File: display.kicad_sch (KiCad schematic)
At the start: 17 parts, among them Q1 ZXM61N03F, U1 E2206KS0E1

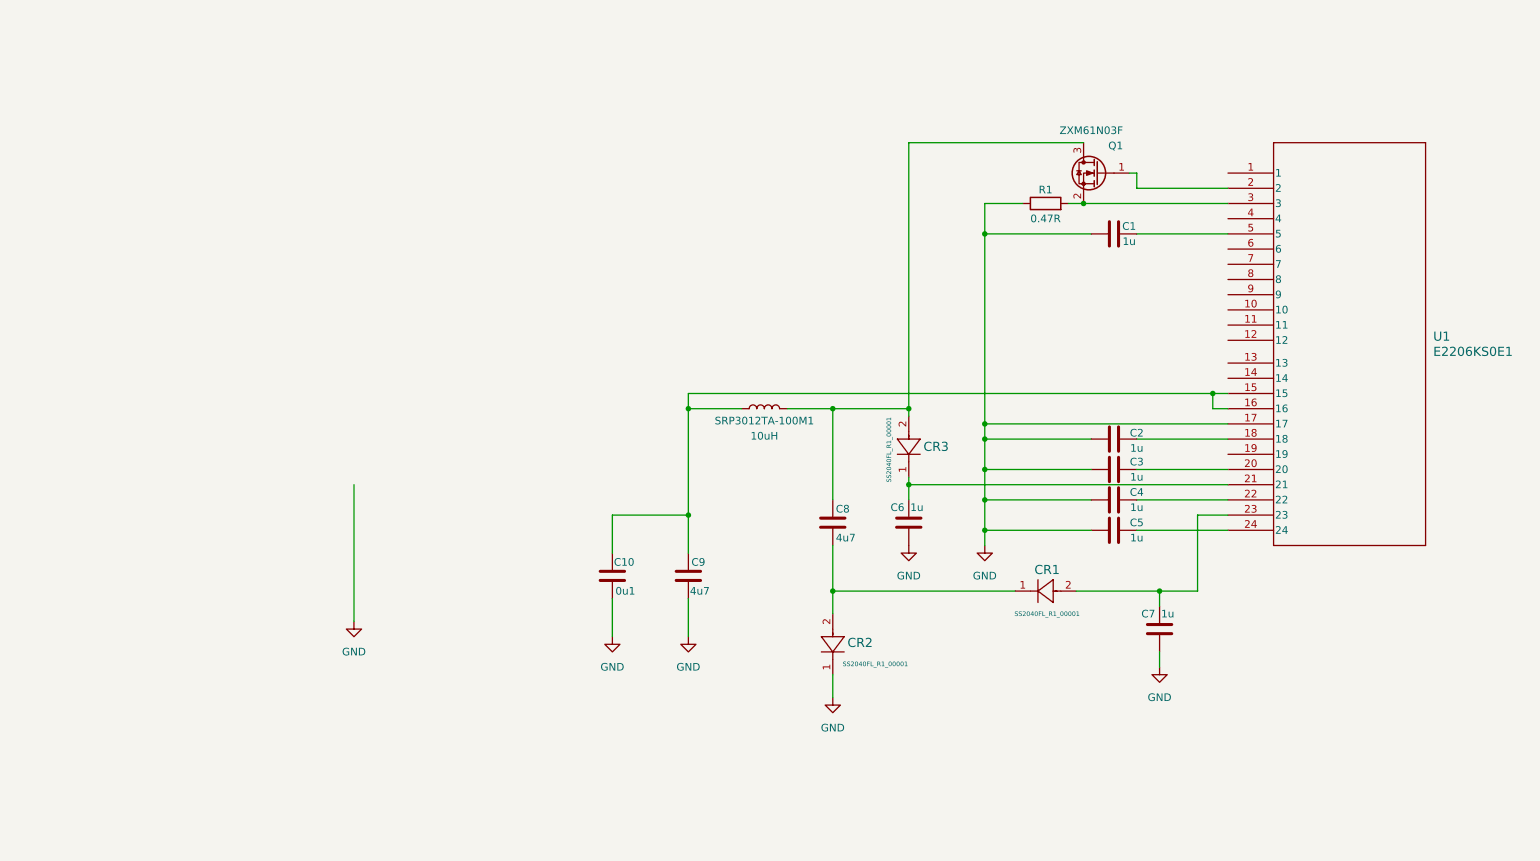
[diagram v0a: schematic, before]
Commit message: .
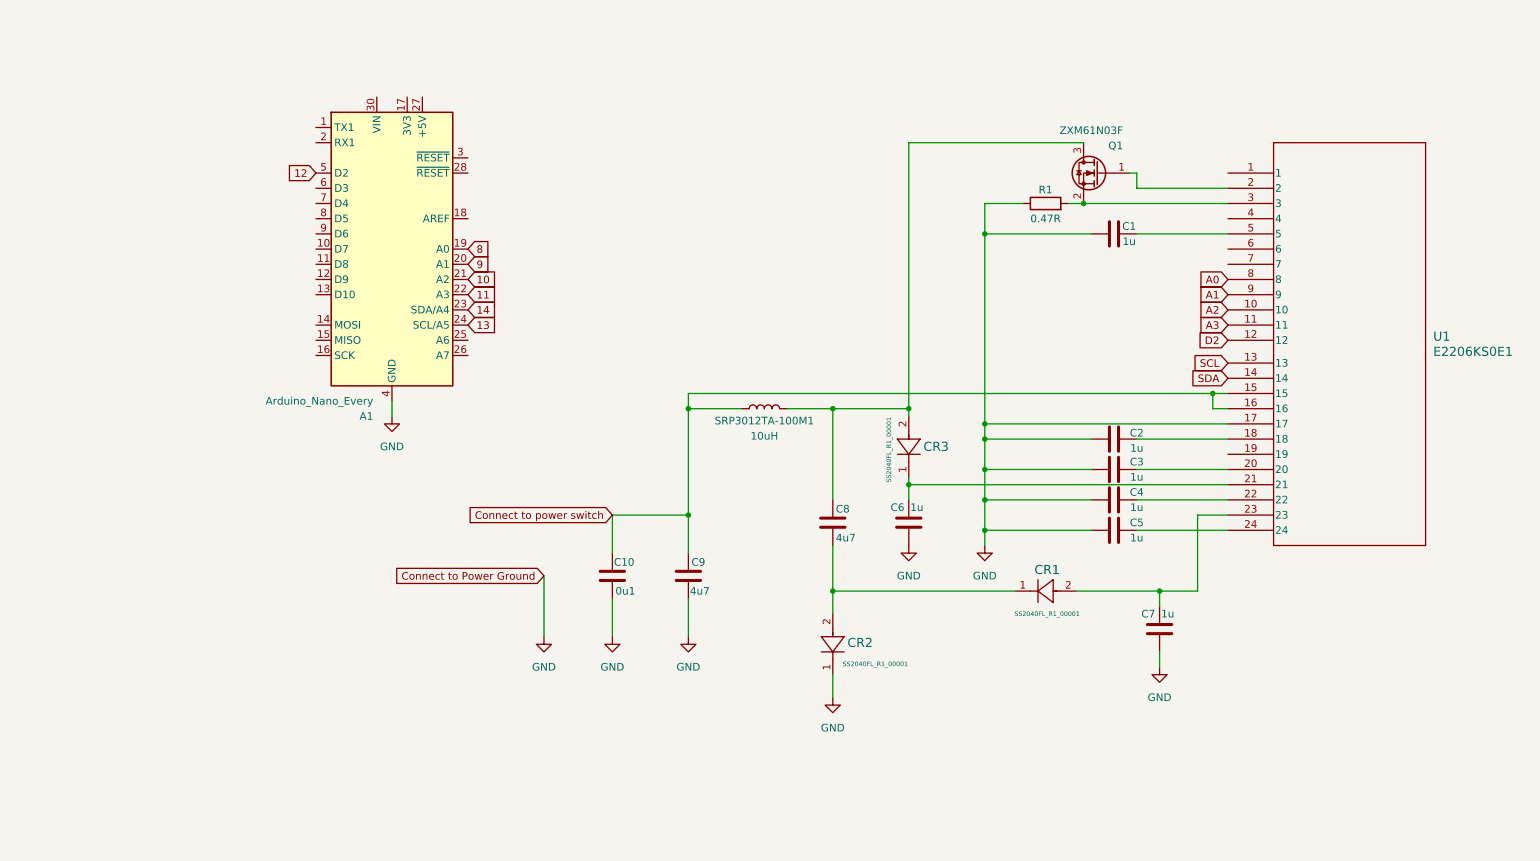
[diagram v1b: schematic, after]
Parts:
- added A1: Arduino_Nano_Every, Module:Arduino_Nano, symbol rsx_Modules:Arduino_Nano_Every
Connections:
- net GND: now also A1.29 (GND), A1.4 (GND)
- net Connect to power switch: now reaches C10.1, C9.1, SRP3012TA-100M1.1, U1.15, U1.16
- net A2: now reaches U1.10
- net A3: now reaches U1.11
- net D2: now reaches U1.12
- net SCL: now reaches U1.13
- net SDA: now reaches U1.14
- net A0: now reaches U1.8
- net A1: now reaches U1.9
- new net 10: A1.21 (A2)
- new net 11: A1.22 (A3)
- new net 12: A1.5 (D2)
- new net 13: A1.24 (SCL/A5)
- new net 14: A1.23 (SDA/A4)
- new net 8: A1.19 (A0)
- new net 9: A1.20 (A1)

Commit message: Nano every
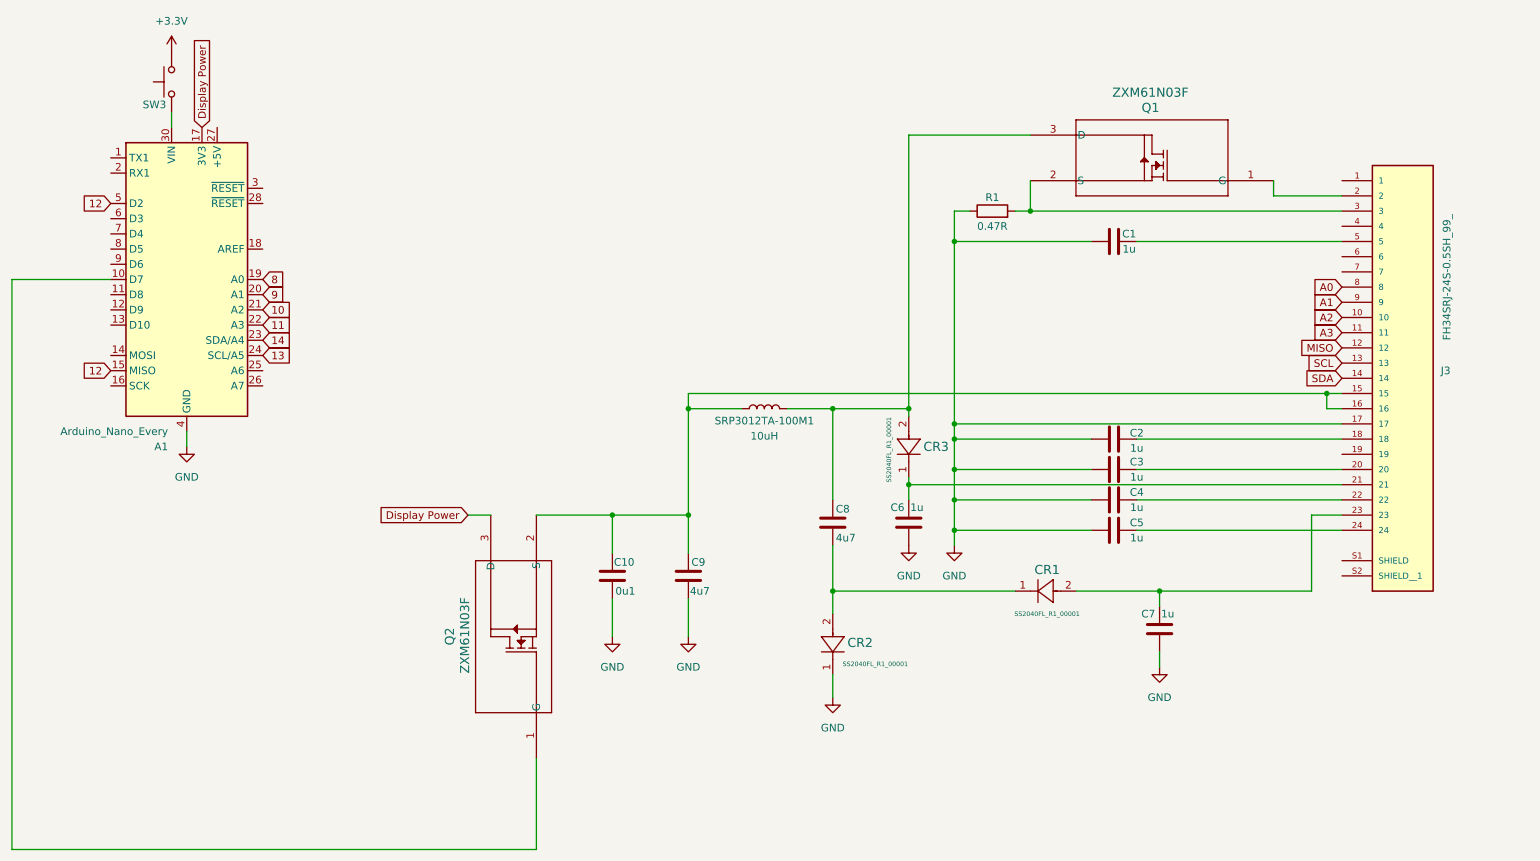
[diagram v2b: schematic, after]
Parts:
- removed Q1: ZXM61N03F, Package_TO_SOT_SMD:SOT-23, symbol Transistor_FET:ZXM61N03F
- removed U1: E2206KS0E1, SOIC_096NL_PUL, symbol rsx_misc:Graphic Display
- added J3: FH34SRJ-24S-0.5SH_99_, rsx_headers_communications:HRS_FH34SRJ-24S-0.5SH_99_, symbol rsx_Header_communication:FH34SRJ-24S-0.5SH_99_
- added Q1, Q2: ZXM61N03F, rsx_packages_TO_SOT:SOT-23, symbol rsx_Transistors:ZXM61N03F
- added SW3: Button-THT - 2-1825910-7, rsx_HID:2-1825910-7, symbol rsx_HID:Button-THT - 2-1825910-7
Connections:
- net 12: now also A1.15 (MISO)
- net A0: now also J3.8
- net A1: now also J3.9
- net A2: now also J3.10
- net A3: now also J3.11
- net GND: now also J3.17
- net SCL: now also J3.13
- net SDA: now also J3.14
- net at C2.2: now also J3.18
- net at C6.2, CR3.1: now also J3.21
- net at R1.2: now also J3.3, Q1.2 (S)
- net at C7.2, CR1.2: now also J3.23
- net at C3.2: now also J3.20
- net at C4.2: now also J3.22
- net at C5.2: now also J3.24
- net at C1.2: now also J3.5
- net at A1.10 (D7): now also Q2.1 (G)
- net Display Power: now reaches A1.17 (3V3)
- net Display Power: now also Q2.3 (D)
- net at A1.30 (VIN): now also SW3.1
- net at C8.1, CR3.2, SRP3012TA-100M1.2: now also Q1.3 (D)
- net Connect to power switch: no longer names the net of C10.1, C9.1, SRP3012TA-100M1.1
- net Connect to power switch: now also J3.15, J3.16, Q2.2 (S)
- new net: J3.2, Q1.1 (G)
- new net +3.3V: SW3.2
- new net MISO: J3.12
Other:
- moved on the sheet: A1, C1, R1
